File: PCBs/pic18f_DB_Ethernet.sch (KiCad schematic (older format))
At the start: 40 parts, among them J1 OC1, J2 PicKIT 3, J3 IC1, J4 FC1, J5 MC1, J6 DB9_Female, J7 DB9_Male, J8 RJ45, SW1 SW_DPDT_x2, SW2 PWR_SW, U1 pic18f45k20

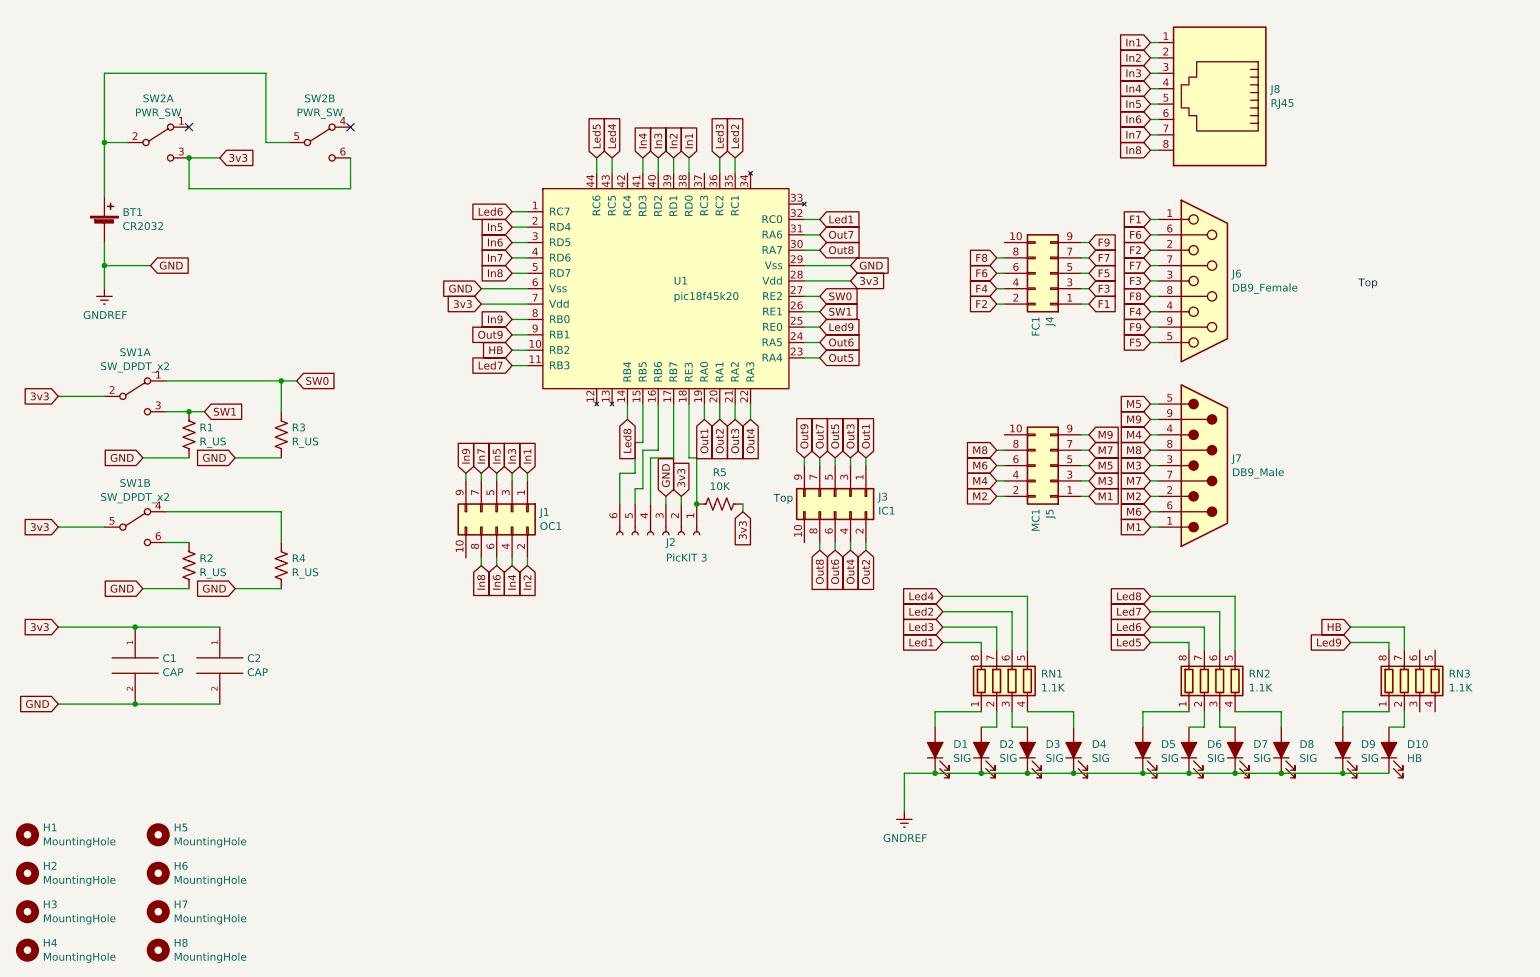
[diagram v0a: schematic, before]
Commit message: Restructed project
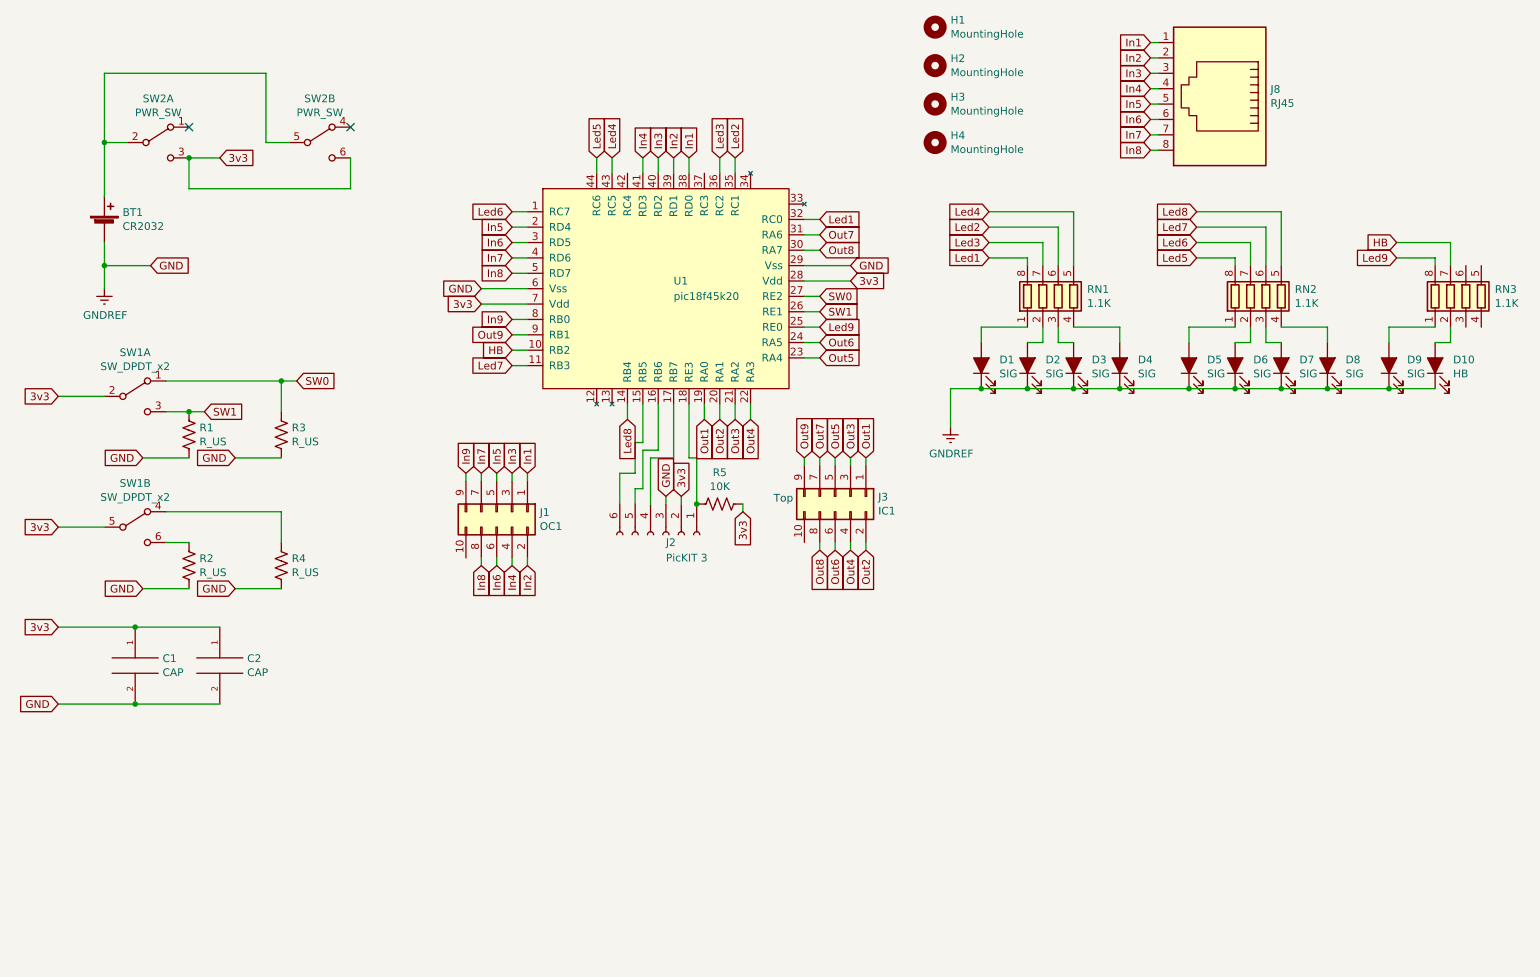
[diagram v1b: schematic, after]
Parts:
- removed H5, H6, H7, H8: MountingHole, MountingHole:MountingHole_3.2mm_M3, symbol Mechanical:MountingHole
- removed J4: FC1, Connector_PinHeader_2.54mm:PinHeader_2x05_P2.54mm_Vertical, symbol Connector_Generic:Conn_02x05_Odd_Even
- removed J5: MC1, Connector_PinHeader_2.54mm:PinHeader_2x05_P2.54mm_Vertical, symbol Connector_Generic:Conn_02x05_Odd_Even
- removed J6: DB9_Female, Connector_Dsub:DSUB-9_Female_Horizontal_P2.77x2.84mm_EdgePinOffset9.90mm_Housed_MountingHolesOffset11.32mm, symbol Connector:DB9_Female
- removed J7: DB9_Male, Connector_Dsub:DSUB-9_Female_Horizontal_P2.77x2.84mm_EdgePinOffset9.90mm_Housed_MountingHolesOffset11.32mm, symbol Connector:DB9_Male
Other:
- moved on the sheet: D1, D10, D2, D3, D4, D5, D6, D7, D8, D9, H1, H2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
